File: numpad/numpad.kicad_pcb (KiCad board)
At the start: 2 copper layers, 81.3 x 110.5 mm, 52 parts, among them SW1 SW_Push, U1 ATmega32U2-A, U2 PRTR5V0U2X, Y1 Crystal_GND24_Small

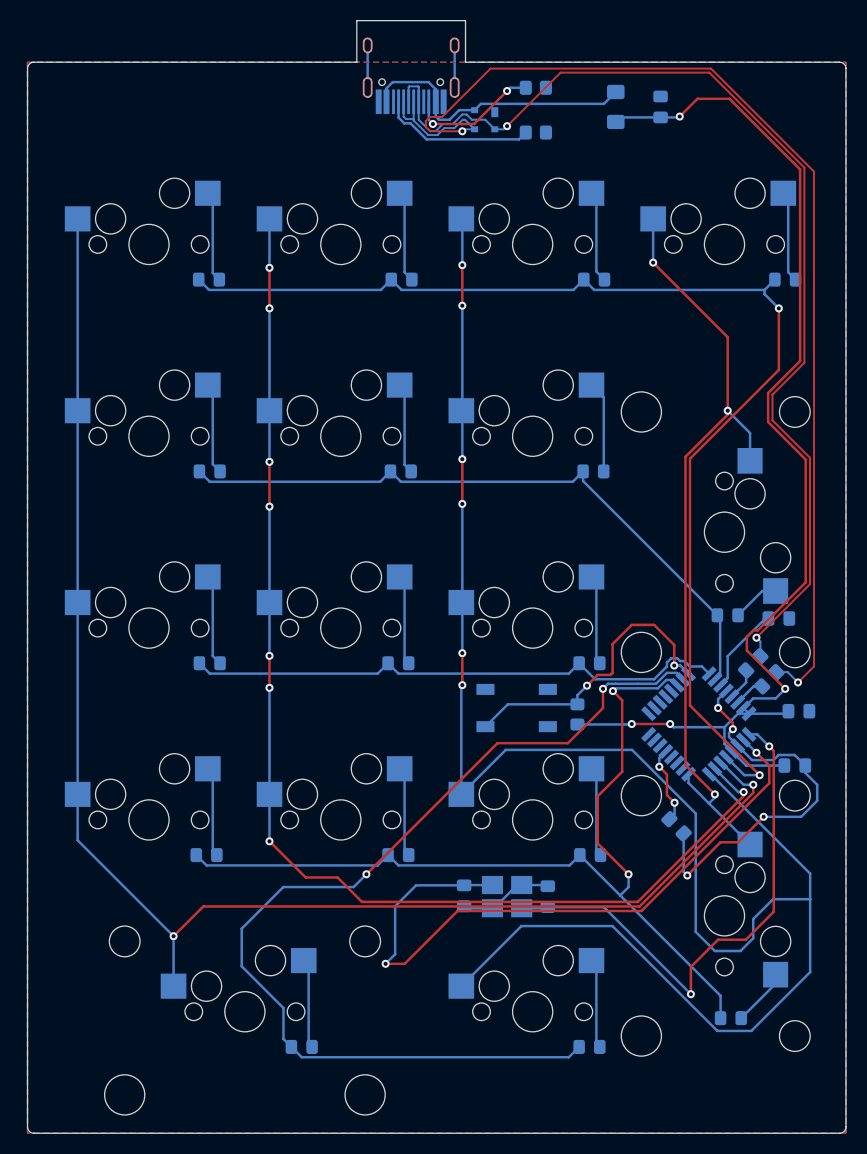
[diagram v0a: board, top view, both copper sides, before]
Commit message: finished numpad pcb
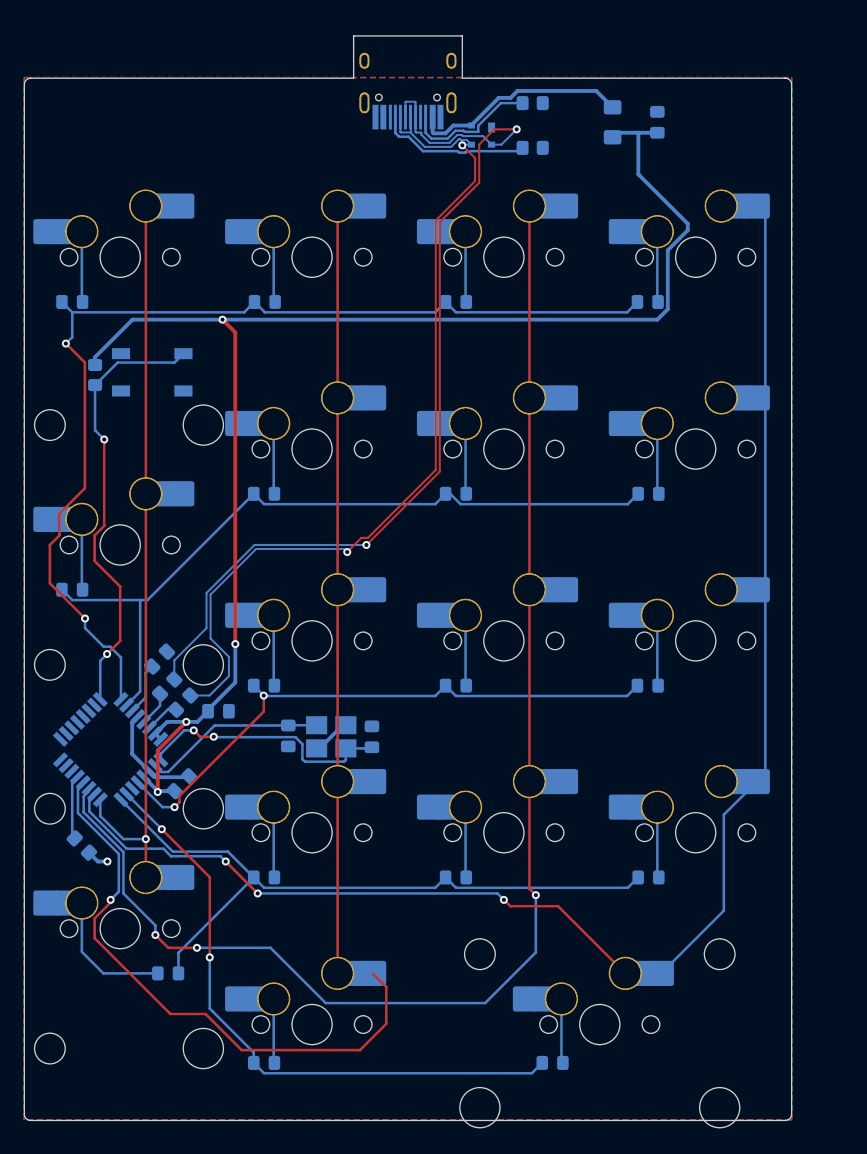
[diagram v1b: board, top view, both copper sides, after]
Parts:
- removed MX1, MX10, MX11, MX12, MX13, MX14, MX17, MX2, MX3, MX4, MX5, MX6, MX7, MX9: MX-NoLED, MX_Only:MXOnly-1U-Hotswap
- removed MX15, MX16, MX8: MX-NoLED, MX_Only:MXOnly-2U-Hotswap
- added S1: MX_stab, marbastlib-mx:STAB_MX_2u, B.Cu at (166.1, 93.0)
- added S2: MX_stab, marbastlib-mx:STAB_MX_2u, B.Cu at (213.7, 140.7)
- added S3: MX_stab, marbastlib-mx:STAB_MX_2u, B.Cu at (166.1, 131.1)
- added SW10: MX_SW_HS, marbastlib-mx:SW_MX_HS_1u, B.Cu at (223.2, 102.6)
- added SW11: MX_SW_HS, marbastlib-mx:SW_MX_HS_1u, B.Cu at (204.2, 102.6)
- added SW12: MX_SW_HS, marbastlib-mx:SW_MX_HS_1u, B.Cu at (185.1, 102.6)
- added SW13: MX_SW_HS, marbastlib-mx:SW_MX_HS_1u, B.Cu at (223.2, 121.6)
- added SW14: MX_SW_HS, marbastlib-mx:SW_MX_HS_1u, B.Cu at (204.2, 121.6)
- added SW15: MX_SW_HS, marbastlib-mx:SW_MX_HS_1u, B.Cu at (185.1, 121.6)
- added SW16: MX_SW_HS, marbastlib-mx:SW_MX_HS_1u, B.Cu at (166.1, 131.1)
- added SW17: MX_SW_HS, marbastlib-mx:SW_MX_HS_1u, B.Cu at (213.7, 140.7)
- added SW18: MX_SW_HS, marbastlib-mx:SW_MX_HS_1u, B.Cu at (185.1, 140.7)
- added SW2: MX_SW_HS, marbastlib-mx:SW_MX_HS_1u, B.Cu at (223.2, 64.5)
- added SW3: MX_SW_HS, marbastlib-mx:SW_MX_HS_1u, B.Cu at (204.2, 64.5)
- added SW4: MX_SW_HS, marbastlib-mx:SW_MX_HS_1u, B.Cu at (185.1, 64.5)
- added SW5: MX_SW_HS, marbastlib-mx:SW_MX_HS_1u, B.Cu at (166.1, 64.5)
- added SW6: MX_SW_HS, marbastlib-mx:SW_MX_HS_1u, B.Cu at (223.2, 83.5)
- added SW7: MX_SW_HS, marbastlib-mx:SW_MX_HS_1u, B.Cu at (204.2, 83.5)
- added SW8: MX_SW_HS, marbastlib-mx:SW_MX_HS_1u, B.Cu at (185.1, 83.5)
- added SW9: MX_SW_HS, marbastlib-mx:SW_MX_HS_1u, B.Cu at (166.1, 93.0)
- moved D4 70.8 mm to (161.3, 68.9)
- moved D8 65.1 mm to (161.3, 97.5)
- moved C1 61.6 mm to (170.0, 104.4), turned to 45 degrees
- moved C4 60.9 mm to (172.2, 116.7), turned to 45 degrees
- moved R6 59.1 mm to (162.2, 122.9)
- moved R1 58.6 mm to (163.6, 76.2), turned to -90 degrees
- moved U1 58.5 mm to (165.1, 113.3)
- moved R2 58.2 mm to (170.7, 107.1)
- moved R3 58.2 mm to (172.3, 108.7)
- moved C5 57.6 mm to (175.8, 109.5)
- moved D17 56.1 mm to (170.8, 135.6), turned to 180 degrees
- moved SW1 49.2 mm to (169.2, 75.9), turned to 180 degrees
- moved D14 43.9 mm to (218.5, 126.0)
- moved D5 43.6 mm to (218.5, 87.9)
- moved D1 43.6 mm to (218.4, 68.9)
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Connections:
- U1 pad 10: unconnected-(U1-Pad10) -> COL0
- U1 pad 11: unconnected-(U1-Pad11) -> COL1
- U1 pad 12: unconnected-(U1-Pad12) -> COL2
- U1 pad 22: ROW3 -> unconnected-(U1-Pad22)
- U1 pad 23: ROW4 -> unconnected-(U1-Pad23)
- U1 pad 25: ROW2 -> ROW0
- U1 pad 5: ROW0 -> ROW2
- U1 pad 6: COL0 -> unconnected-(U1-Pad6)
- U1 pad 7: COL1 -> ROW4
- U1 pad 8: COL2 -> ROW3
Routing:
- net XTAL2: track 67.5 -> 18.2 mm, vias 2 -> 0
- net COL2: track 179.3 -> 134.7 mm, vias 6 -> 1
- net GND: track 56.9 -> 16.7 mm, vias 4 -> 1
- net ROW4: track 98.9 -> 61.4 mm
- net D-: track 116.7 -> 87.8 mm
- net +5V: track 116.8 -> 144.1 mm
- net XTAL1: track 52.7 -> 26.1 mm
- net ROW3: track 92.1 -> 68.9 mm, vias 2 -> 0
- net ROW0: track 119.1 -> 103.9 mm
- net COL1: track 120.0 -> 134.8 mm, vias 8 -> 3
- net Net-(R1-Pad2): track 29.8 -> 43.9 mm
- net D+: track 105.8 -> 94.0 mm
- net ROW1: track 66.8 -> 74.7 mm
- net Net-(D17-Pad2): track 5.73 -> 13.3 mm
- net VCC: track 28.6 -> 21.9 mm
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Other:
- board size 81.3 x 110.5 mm -> 76.2 x 107.7 mm

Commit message: did a bit of work 3d modelling today
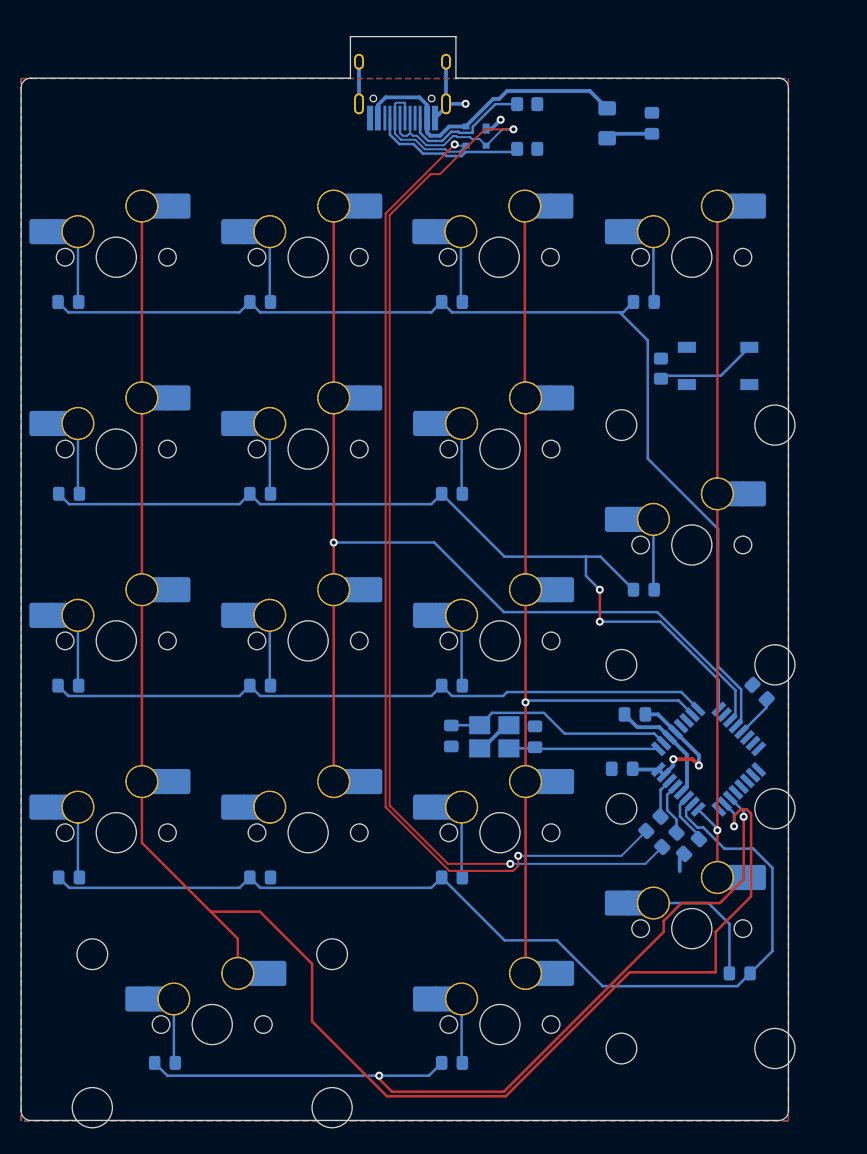
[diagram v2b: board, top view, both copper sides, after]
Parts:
- moved R6 69.0 mm to (229.6, 107.6), turned to 135 degrees
- moved U1 59.4 mm to (224.5, 114.3), turned to -45 degrees
- moved D14 57.5 mm to (161.0, 126.0)
- moved D5 57.5 mm to (161.0, 87.9)
- moved D9 57.5 mm to (160.9, 107.0)
- moved SW10 57.5 mm to (165.7, 102.6)
- moved SW13 57.5 mm to (165.7, 121.6)
- moved SW6 57.5 mm to (165.7, 83.5)
- moved D1 57.5 mm to (160.9, 68.9)
- moved SW2 57.5 mm to (165.7, 64.5)
- moved D17 56.8 mm to (227.6, 135.6)
- moved S3 56.8 mm to (222.8, 131.1)
- moved SW16 56.8 mm to (222.8, 131.1)
- moved D4 56.8 mm to (218.1, 68.9)
- moved D8 56.8 mm to (218.1, 97.5)
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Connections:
- U1 pad 10: COL0 -> unconnected-(U1-Pad10)
- U1 pad 12: COL2 -> ROW0
- U1 pad 22: unconnected-(U1-Pad22) -> ROW4
- U1 pad 23: unconnected-(U1-Pad23) -> COL0
- U1 pad 25: ROW0 -> COL3
- U1 pad 26: ROW1 -> ROW3
- U1 pad 5: ROW2 -> unconnected-(U1-Pad5)
- U1 pad 7: ROW4 -> COL2
- U1 pad 8: ROW3 -> ROW2
- U1 pad 9: COL3 -> ROW1
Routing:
- net +5V: track 144.1 -> 21.0 mm, vias 4 -> 2
- net COL2: track 134.7 -> 93.5 mm
- net Net-(R1-Pad2): track 43.9 -> 10.1 mm, vias 2 -> 0
- net ROW3: track 68.9 -> 99.0 mm
- net COL1: track 134.8 -> 106.3 mm, vias 3 -> 1
- net D+: track 94.0 -> 121.0 mm
- net D-: track 87.8 -> 114.1 mm
- net COL0: track 144.0 -> 169.3 mm, vias 3 -> 1
- net ROW4: track 61.4 -> 84.6 mm
- net GND: track 16.7 -> 31.6 mm, vias 1 -> 2
- net ROW1: track 74.7 -> 86.8 mm, vias 0 -> 2
- net XTAL1: track 26.1 -> 15.0 mm, vias 2 -> 0
- net VCC: track 21.9 -> 30.1 mm
- net ROW2: track 59.2 -> 66.6 mm, vias 2 -> 0
- net Net-(D15-Pad2): track 7.02 -> 0.00 mm
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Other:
- board size 76.2 x 107.7 mm -> 76.2 x 107.6 mm

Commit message: work
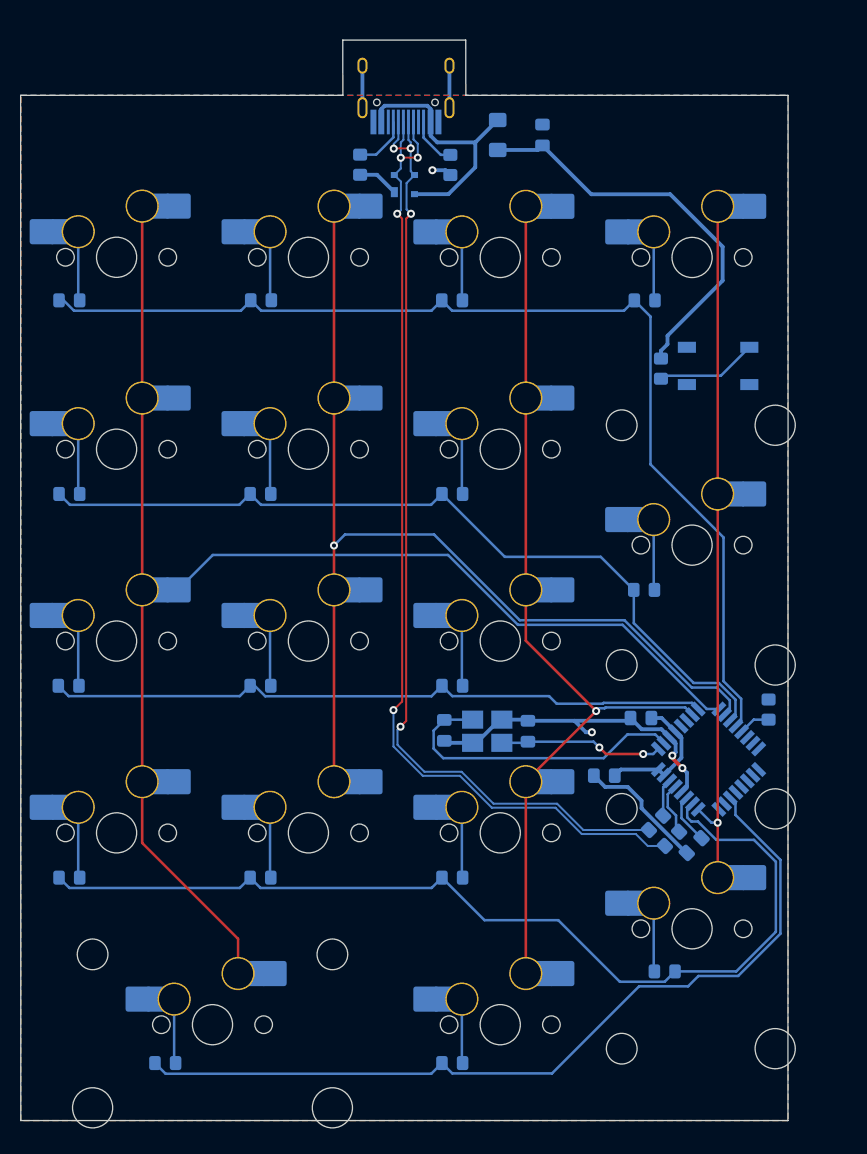
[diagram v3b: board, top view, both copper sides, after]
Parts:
- moved R4 16.7 mm to (189.9, 55.3), turned to 90 degrees
- moved C6 10.9 mm to (208.0, 52.3)
- moved F1 10.9 mm to (203.5, 52.3)
- moved R5 9.73 mm to (198.8, 55.3), turned to 90 degrees
- moved U2 8.59 mm to (194.3, 57.2), turned to 0 degrees
- moved D15 7.45 mm to (220.1, 135.4)
- moved R6 1.95 mm to (230.4, 109.4), turned to 90 degrees
- moved C5 1.90 mm to (214.1, 115.9)
- moved C2 0.89 mm to (206.5, 111.5)
- moved C3 0.89 mm to (198.2, 111.4)
- moved Y1 0.89 mm to (202.5, 111.5)
- moved C4 0.69 mm to (217.8, 110.2)
- moved USB1 0.52 mm to (194.4, 42.8)
- moved C1 0.28 mm to (223.0, 122.9)
- moved R2 0.28 mm to (220.8, 122.2)
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- renumbered D14 to D12, D15 to D13, D16 to D14, D17 to D15, D18 to D16, D19 to D17, SW2 to SW1, SW11 to SW10, SW12 to SW11, SW13 to SW12, SW14 to SW13, SW15 to SW14, SW16 to SW15, SW17 to SW16, SW18 to SW17, SW1 to SW18, SW3 to SW2, SW4 to SW3, SW5 to SW4, SW6 to SW5, SW7 to SW6, SW8 to SW7, SW9 to SW8, SW10 to SW9
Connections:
- U1 pad 10: unconnected-(U1-Pad10) -> COL1
- U1 pad 11: COL1 -> ROW1
- U1 pad 23: COL0 -> unconnected-(U1-Pad23)
- U1 pad 9: ROW1 -> COL0
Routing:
- net +5V: track 21.0 -> 53.9 mm, vias 2 -> 0
- net GND: track 31.6 -> 59.5 mm, vias 2 -> 4
- net COL0: track 169.3 -> 141.6 mm, vias 1 -> 0
- net D+: track 121.0 -> 99.8 mm, vias 2 -> 4
- net D-: track 114.1 -> 96.2 mm, vias 2 -> 4
- net Net-(R4-Pad2): track 15.5 -> 5.54 mm
- net Net-(R5-Pad2): track 13.4 -> 4.92 mm
- net XTAL2: track 22.9 -> 30.7 mm
- net Net-(D13-Pad2): track 0.00 -> 7.02 mm
- net Net-(D15-Pad2): track 13.3 -> 6.80 mm
- net ROW1: track 86.8 -> 81.6 mm, vias 2 -> 0
- net VCC: track 30.1 -> 26.6 mm
- net COL2: track 93.5 -> 92.0 mm
- net XTAL1: track 15.0 -> 16.1 mm, vias 0 -> 2
- net Net-(R6-Pad1): track 4.31 -> 3.18 mm
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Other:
- board size 76.2 x 107.6 mm -> 76.2 x 107.3 mm
